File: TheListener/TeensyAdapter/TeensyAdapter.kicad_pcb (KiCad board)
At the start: 2 copper layers, 61 x 36.8 mm, 21 parts, among them J1 Conn_02x05_Odd_Even, J2 Conn_02x05_Odd_Even, J3 Conn_02x02_Odd_Even, U1 Teensy3.5

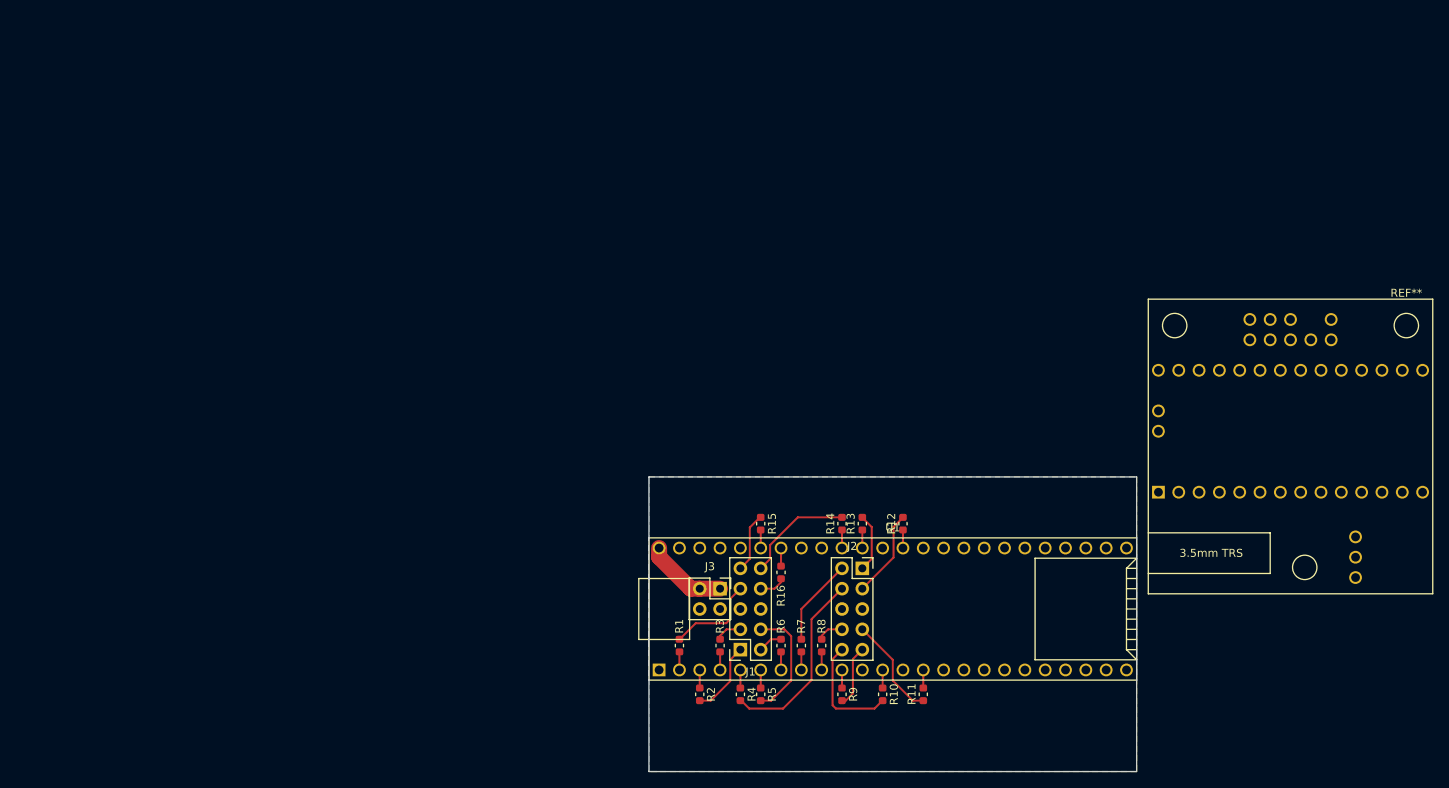
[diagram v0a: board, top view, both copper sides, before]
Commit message: update
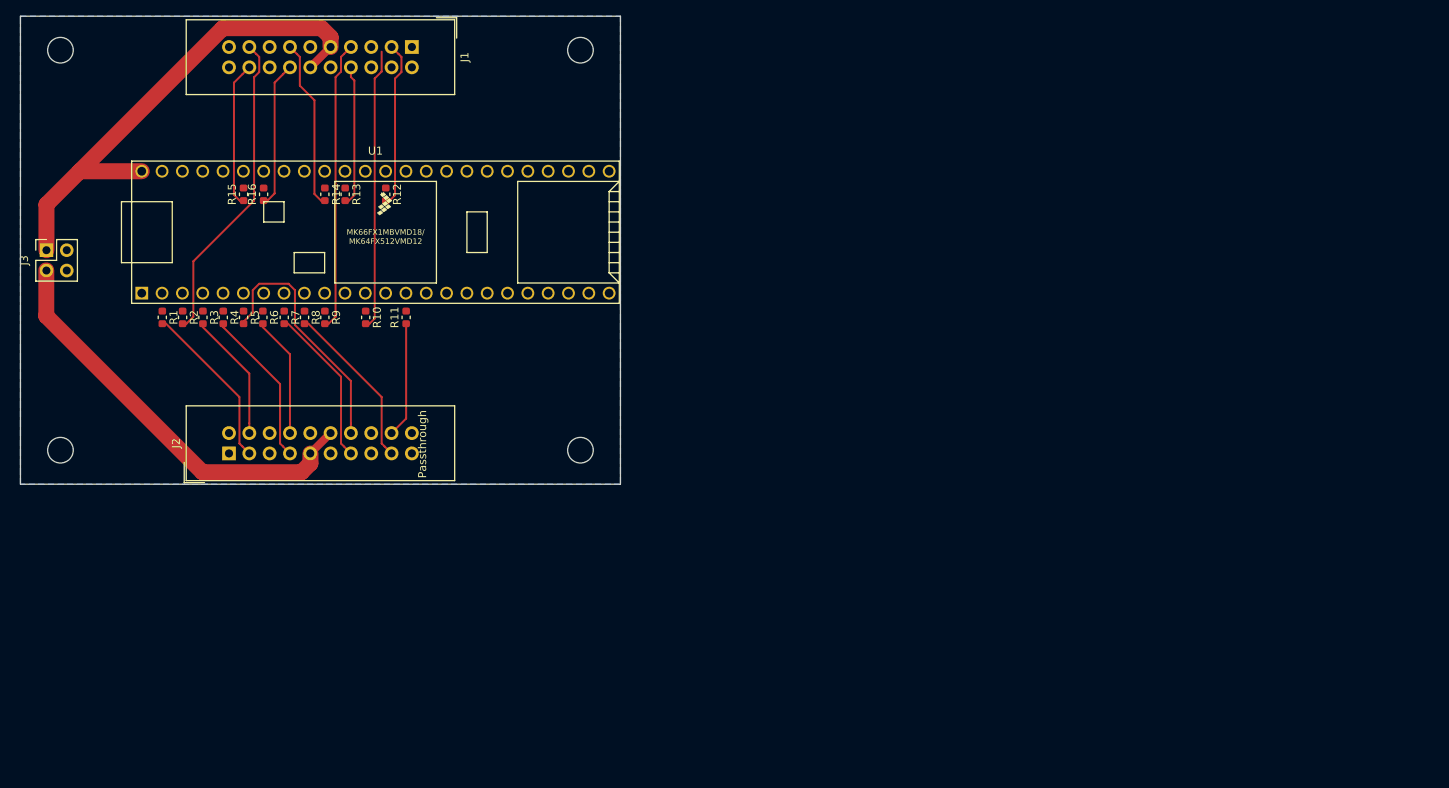
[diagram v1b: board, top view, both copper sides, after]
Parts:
- removed REF**: TeensyAudioShield, TheListener:TeensyAudioShield
- added H1: MountingHole, MountingHole:MountingHole_3.2mm_M3, F.Cu at (65.5, 63.5)
- added H2: MountingHole, MountingHole:MountingHole_3.2mm_M3, F.Cu at (130.5, 63.5)
- added H3: MountingHole, MountingHole:MountingHole_3.2mm_M3, F.Cu at (130.5, 113.5)
- added H4: MountingHole, MountingHole:MountingHole_3.2mm_M3, F.Cu at (65.5, 113.5)
- J1, J2: value Conn_02x05_Odd_Even -> Conn_02x10_Odd_Even; footprint TheListener:PinSocket_2x05_P2.54mm_Vertical_MinCrtYd -> Connector_IDC:IDC-Header_2x10_P2.54mm_Vertical
- J3: footprint TheListener:PinSocket_2x02_P2.54mm_Vertical_MinCrtYd -> Connector_PinSocket_2.54mm:PinSocket_2x02_P2.54mm_Vertical
- moved J3 94.2 mm to (63.8, 88.5), turned to 90 degrees
- moved J1 85.8 mm to (109.4, 63.1), turned to 270 degrees
- moved J2 80.5 mm to (86.6, 113.9), turned to 90 degrees
- moved R16 80.1 mm to (90.9, 81.5)
- moved U1 80.0 mm to (104.9, 86.2)
- moved R4 80.0 mm to (85.9, 96.9)
- moved R5 80.0 mm to (88.4, 96.9)
- moved R11 80.0 mm to (108.7, 96.9)
- moved R2 80.0 mm to (80.8, 96.9)
- moved R9 80.0 mm to (98.6, 96.9)
- moved R10 80.0 mm to (103.7, 96.9)
- moved R6 76.7 mm to (90.8, 96.9), turned to 270 degrees
- moved R12 76.6 mm to (106.2, 81.5), turned to 270 degrees
- moved R15 76.6 mm to (88.4, 81.5), turned to 90 degrees
- moved R13 76.6 mm to (101.1, 81.5), turned to 270 degrees
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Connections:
- J1 pad 1: R_5 -> GND
- J1 pad 10: R_3 -> GND
- J1 pad 2: T_6 -> GND
- J1 pad 4: R_6 -> R_5
- J1 pad 7: R_4 -> T_6
- J1 pad 8: T_3 -> R_6
- J1 pad 9: T_4 -> +5V
- J2 pad 1: R_1 -> GND
- J2 pad 10: R_7 -> GND
- J2 pad 2: T_2 -> GND
- J2 pad 3: T_1 -> R_4
- J2 pad 4: R_2 -> T_4
- J2 pad 7: R_8 -> R_3
- J2 pad 8: T_7 -> T_3
- J2 pad 9: T_8 -> +5V
- R10 pad 2: R_7 -> R_5
- R11 pad 1: R_8 -> R_1
- R12 pad 2: T_1 -> T_5
- R13 pad 2: R_1 -> R_6
- R14 pad 2: R_3 -> R_7
- R15 pad 1: T_4 -> T_8
- R16 pad 1: T_3 -> T_7
- R2 pad 2: R_5 -> R_8
- R3 pad 2: T_5 -> T_4
- R4 pad 2: R_2 -> R_3
- R5 pad 2: R_6 -> R_2
- R6 pad 2: T_6 -> T_3
- R8 pad 2: T_7 -> T_1
- R9 pad 2: T_8 -> T_6
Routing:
- net +5V: track 10.4 -> 115.5 mm
- net T_6: track 3.08 -> 36.2 mm
- net R_8: track 12.8 -> 39.3 mm
- net R_5: track 9.18 -> 35.1 mm
- net T_5: track 3.31 -> 20.8 mm
- net T_7: track 3.57 -> 18.3 mm
- net T_3: track 3.31 -> 15.1 mm
- net T_8: track 7.71 -> 18.2 mm
- net T_1: track 11.0 -> 21.0 mm
- net R_4: track 11.7 -> 21.0 mm
- net T_2: track 11.0 -> 19.9 mm
- net T_4: track 7.49 -> 16.1 mm
- net R_1: track 6.63 -> 14.4 mm
- net R_2: track 23.8 -> 31.4 mm
- net R_7: track 14.3 -> 21.3 mm
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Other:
- board size 61 x 36.8 mm -> 75 x 58.5 mm
- board text added: "Passthrough"

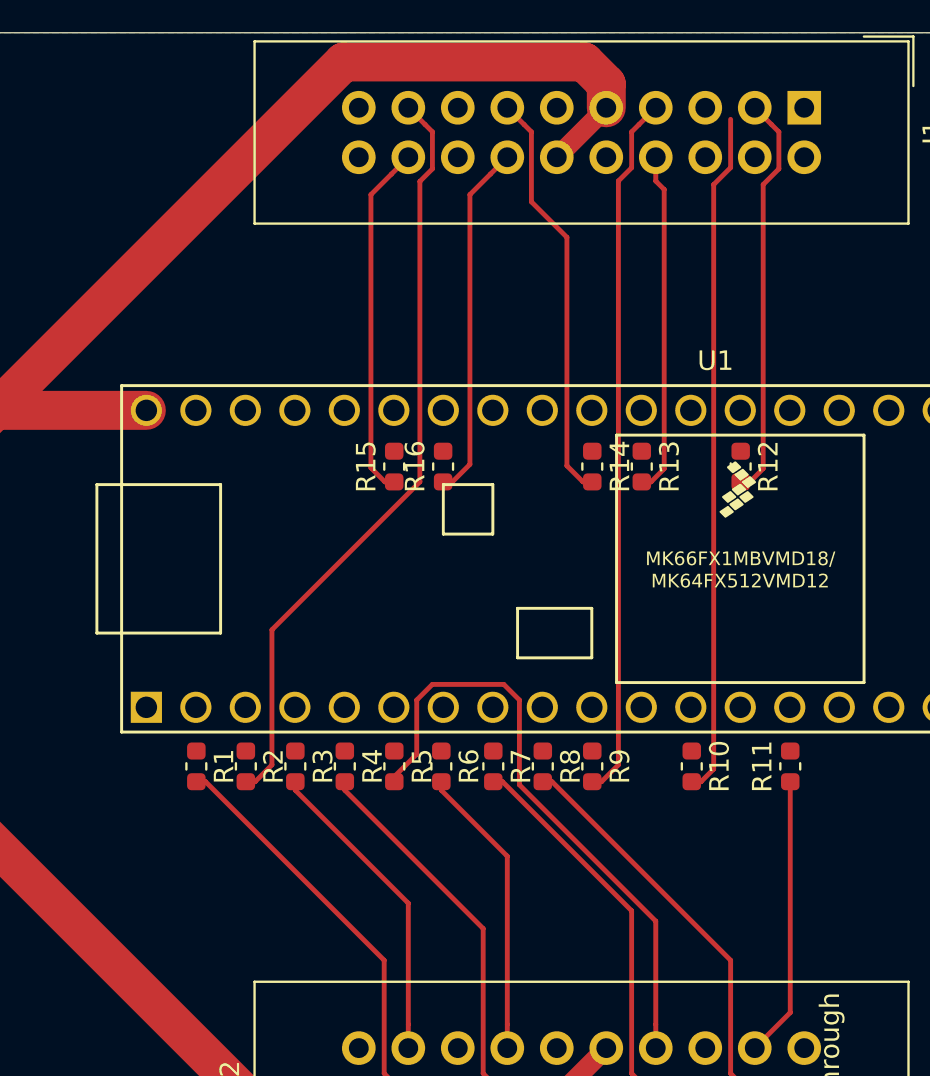
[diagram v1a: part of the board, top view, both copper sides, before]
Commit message: updates
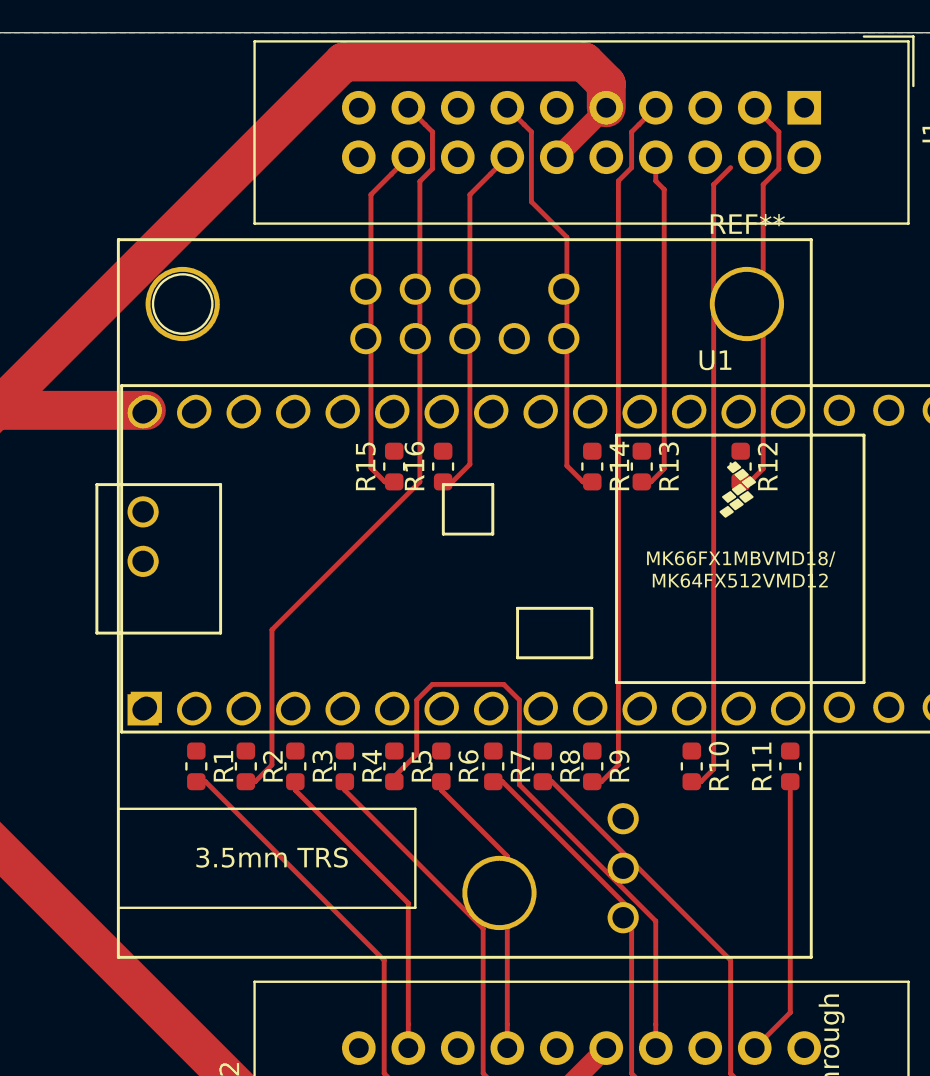
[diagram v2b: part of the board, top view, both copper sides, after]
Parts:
- added REF**: TeensyAudioShield, TheListener:TeensyAudioShield, F.Cu at (75.5, 94.0)
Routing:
- net R_5: track 35.1 -> 32.6 mm
